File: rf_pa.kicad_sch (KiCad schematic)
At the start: 43 parts, among them Q1 BSS138, Q2 NP100P04PDG, U1 LM317_SOT-223, U2 LT1013DIDR, U3 TL431, U4 RA60H3847H1

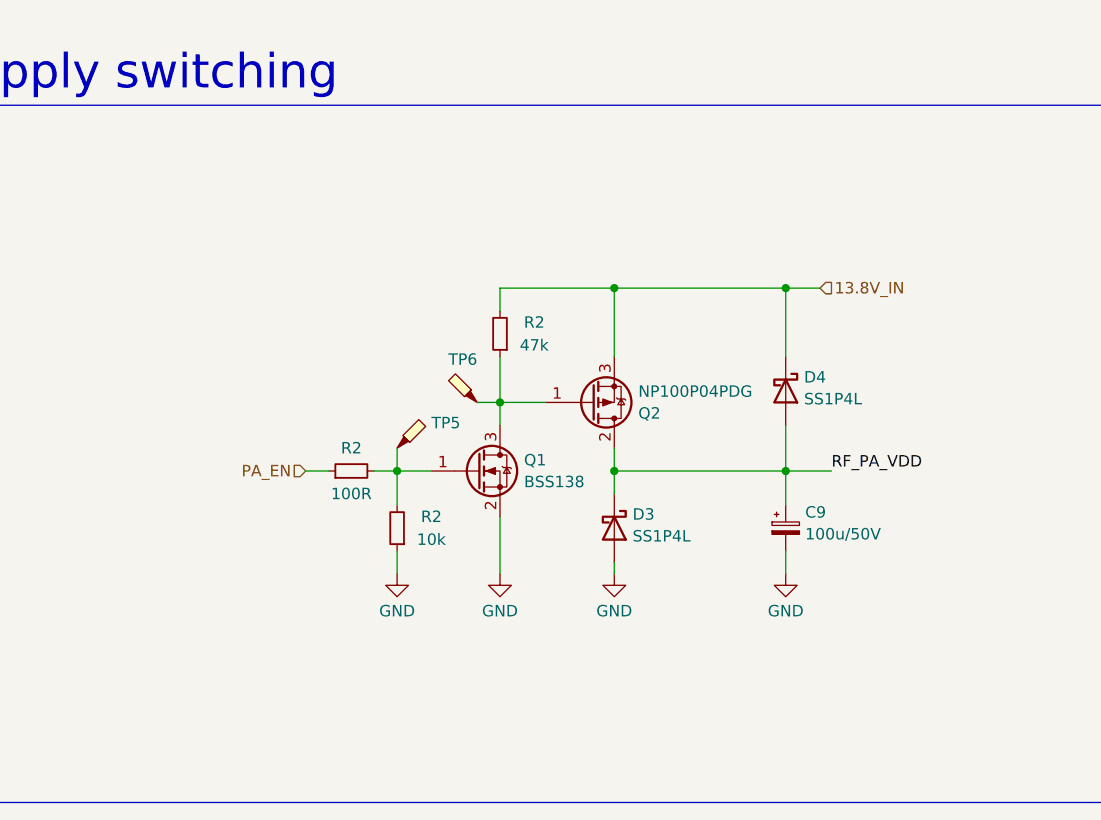
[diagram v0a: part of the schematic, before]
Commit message: Add files via upload
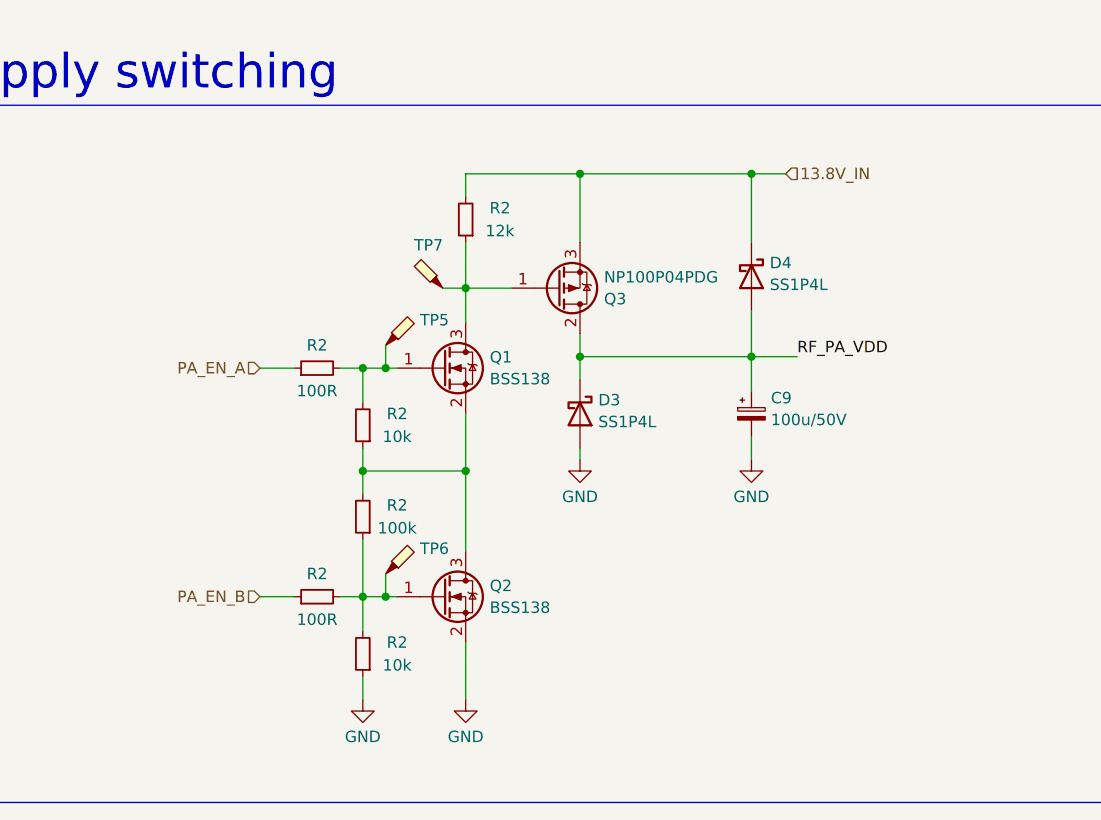
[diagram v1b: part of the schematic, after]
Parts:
- added Q1: BSS138, Package_TO_SOT_SMD:SOT-23, symbol Transistor_FET:BSS138
- added R2: 100k, Resistor_SMD:R_0603_1608Metric, symbol Device:R_Small
- added R2: 100R, Resistor_SMD:R_0603_1608Metric, symbol Device:R_Small
- added R2: 10k, Resistor_SMD:R_0603_1608Metric, symbol Device:R_Small
- added TP5: ~, TestPoint:TestPoint_Pad_D1.5mm, symbol Connector:TestPoint_Probe
- Q2: renamed from Q1; PN (none) -> BSS138P,215
- R2: value 47k -> 12k
- renumbered Q2 to Q3, TP5 to TP6, TP6 to TP7
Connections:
- net at Q2.1 (G), R2.2, R2.2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: now also R2.1
- net at Q3.1 (G), R2.1, TP7.1: now also Q1.3 (D); no longer Q2.3 (D)
- net PA_EN renamed PA_EN_B
- new net: Q1.2 (S), Q2.3 (D), R2.1, R2.2
- new net: Q1.1 (G), R2.2, R2.2, TP5.1
- new net PA_EN_A: R2.1
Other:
- moved on the sheet: C9, D3, D4, Q2, Q3, R2, TP6, TP7
